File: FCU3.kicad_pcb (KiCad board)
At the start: 4 copper layers, 37 x 37 mm, 60 parts, among them J1 SM06B-SRSS-TB(LF)(SN), J2 SM08B-SRSS-TB(LF)(SN), J3 UJ20-C-H-G-SMT-1-P16-TR, J5 SM06B-SRSS-TB(LF)(SN), Q1 SS8050, U1 MPU-6500, U2 AP7375-33SA-7, U3 STM32F405RGT6, Y1 12MHz

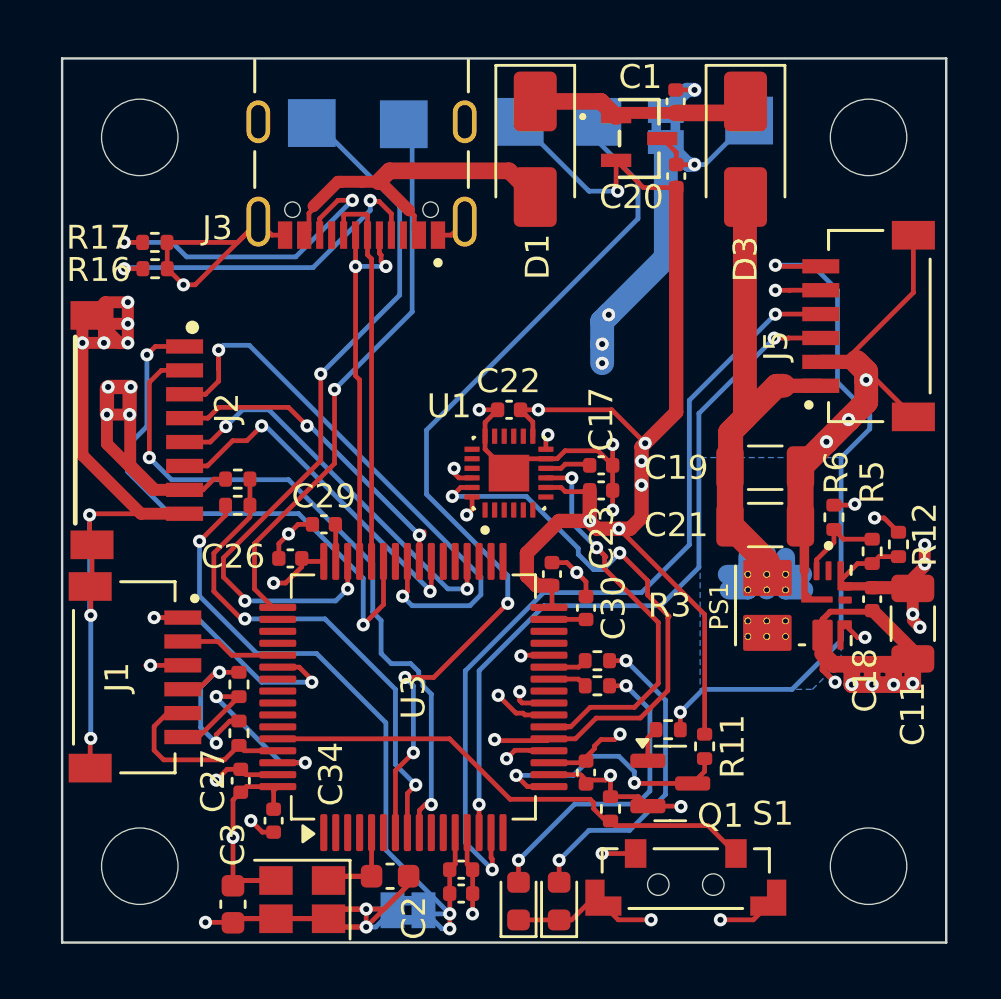
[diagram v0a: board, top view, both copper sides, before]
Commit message: Fix Drawings
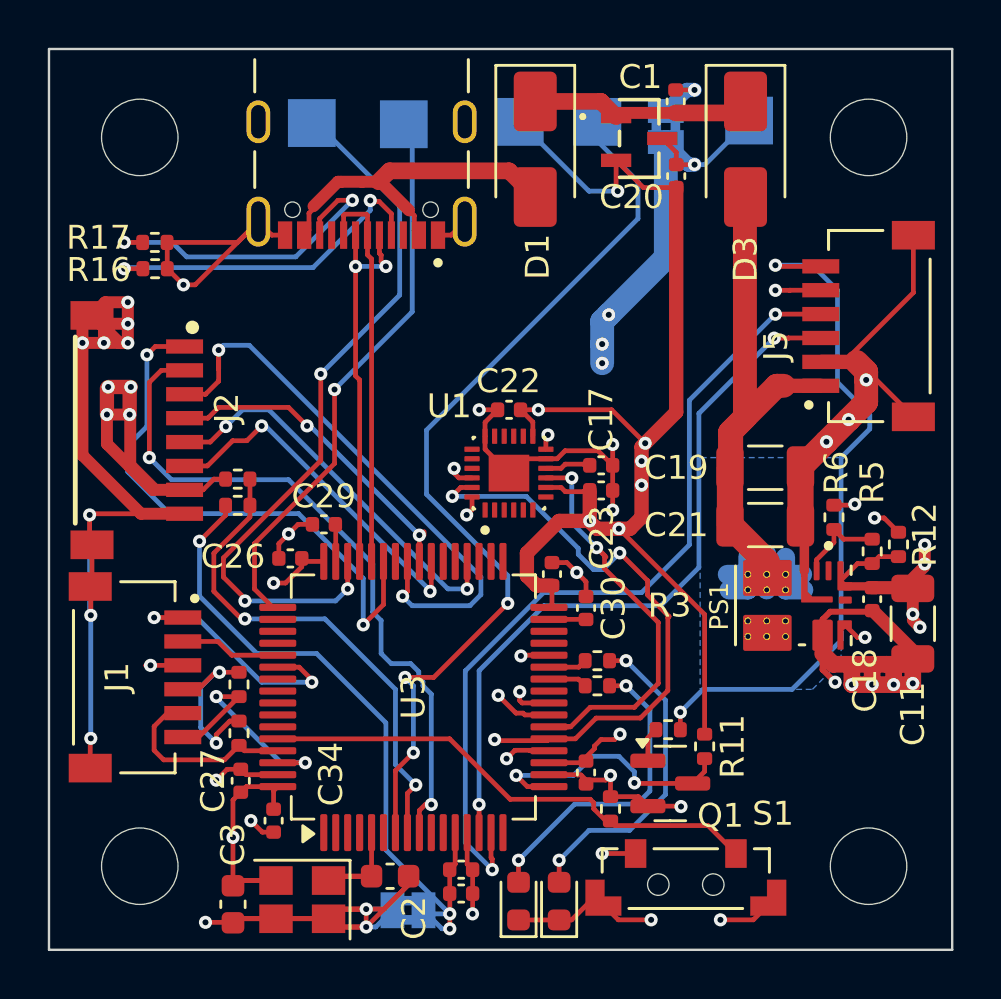
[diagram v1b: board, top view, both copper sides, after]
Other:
- board size 37 x 37 mm -> 37.8 x 37.7 mm
